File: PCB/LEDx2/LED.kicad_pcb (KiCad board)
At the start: 2 copper layers, 70 x 70 mm, 32 parts, among them J1 Reset, J2 Wago, J3 TC2030-USB-NL-DS, J4 Wago, J5 USB-C-Socket-H, J6 Wago, J7 Wago, U6 ESP32-S3-MINI-1, U7 MD8942

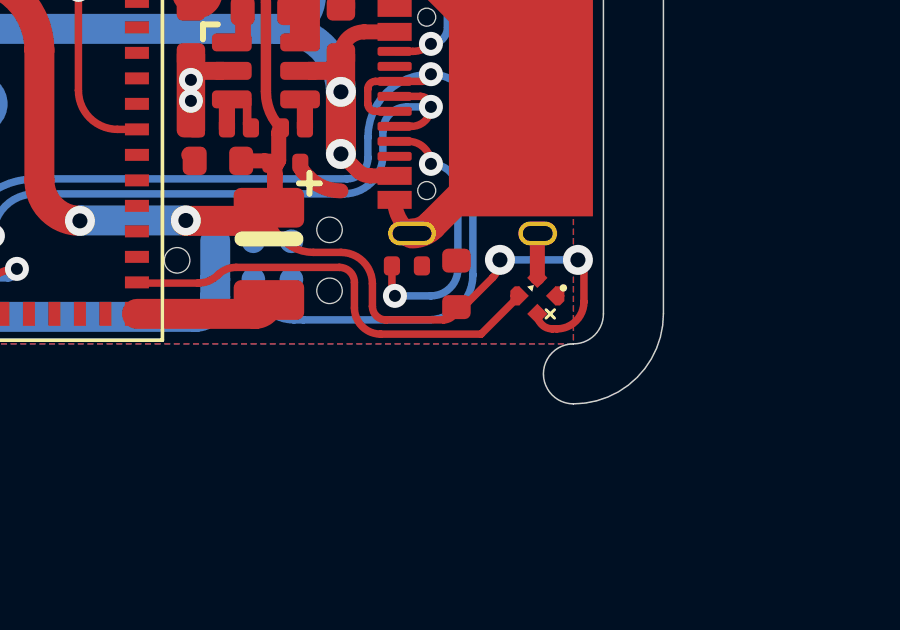
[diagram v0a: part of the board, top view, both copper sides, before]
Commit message: BOM fix
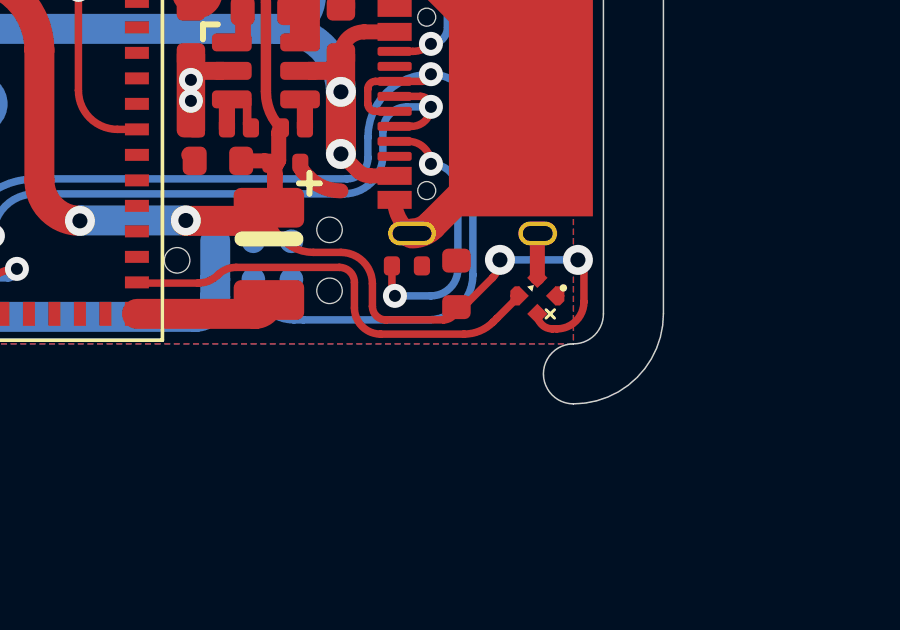
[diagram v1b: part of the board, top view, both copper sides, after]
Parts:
- C10: value 10uF 50V -> 10uF 35V
